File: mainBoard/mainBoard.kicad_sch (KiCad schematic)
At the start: 20 parts, among them J1 Conn_01x01, J2 Conn_01x01, J3 Conn_01x01, J4 Conn_01x01, J5 Conn_01x01, J6 Conn_01x01, J7 Conn_01x01, J8 Conn_01x01, J9 Conn_01x01

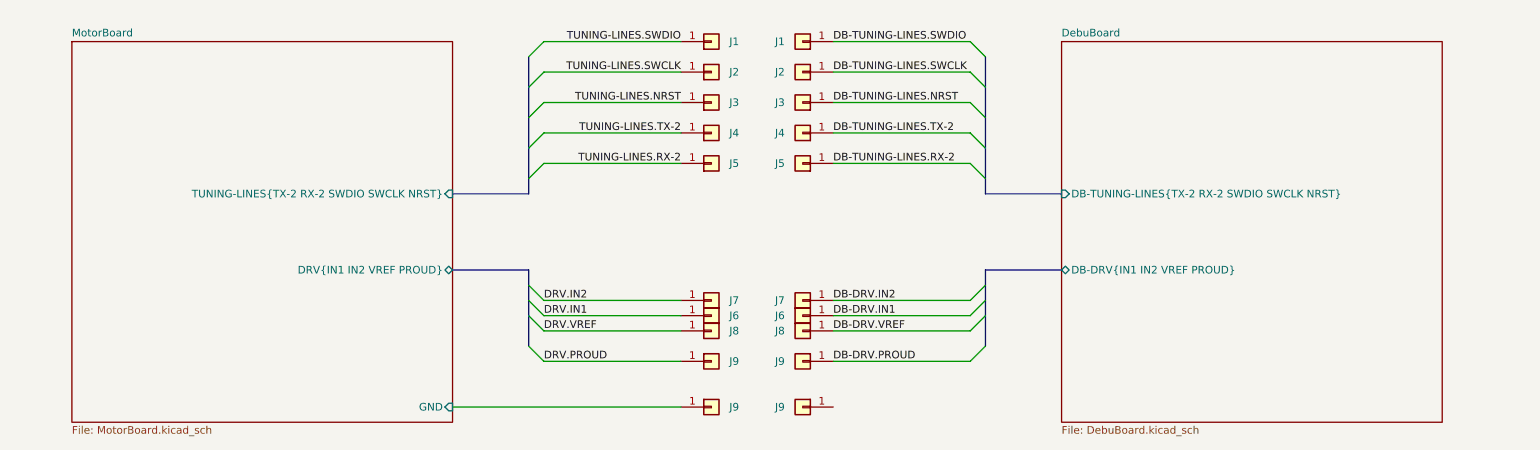
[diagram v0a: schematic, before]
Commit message: DebugBoard
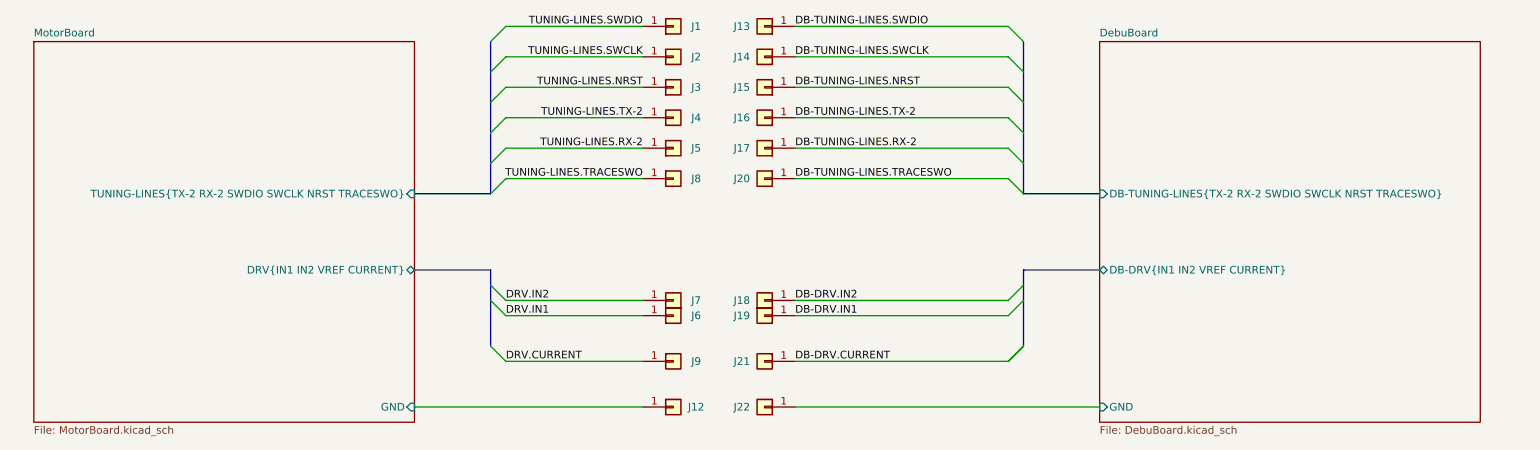
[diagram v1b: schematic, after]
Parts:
- renumbered J9 to J12, J1 to J13, J2 to J14, J3 to J15, J4 to J16, J5 to J17, J7 to J18, J6 to J19, J8 to J20, J9 to J21, J9 to J22
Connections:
- net DebuBoard/GND: now reaches J22.1 (Pin_1)
- net DB-DRV.PROUD renamed DB-DRV.CURRENT
- net DB-DRV.VREF renamed DB-TUNING-LINES.TRACESWO
- net DRV.PROUD renamed DRV.CURRENT
- net DRV.VREF renamed TUNING-LINES.TRACESWO
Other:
- sheet DebuBoard ports: added DB-DRV{IN1 IN2 VREF CURRENT}, DB-TUNING-LINES{TX-2 RX-2 SWDIO SWCLK NRST TRACESWO}, GND; removed DB-DRV{IN1 IN2 VREF PROUD}, DB-TUNING-LINES{TX-2 RX-2 SWDIO SWCLK NRST}
- sheet MotorBoard ports: added DRV{IN1 IN2 VREF CURRENT}, TUNING-LINES{TX-2 RX-2 SWDIO SWCLK NRST TRACESWO}; removed DRV{IN1 IN2 VREF PROUD}, TUNING-LINES{TX-2 RX-2 SWDIO SWCLK NRST}
- moved on the sheet: J1, J12, J13, J14, J15, J16, J17, J18, J19, J2, J20, J21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
